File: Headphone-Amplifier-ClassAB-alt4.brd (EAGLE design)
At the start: 40.6 x 25.4 mm, 17 parts, among them T1 BC547, T2 BC557, T3 BC547

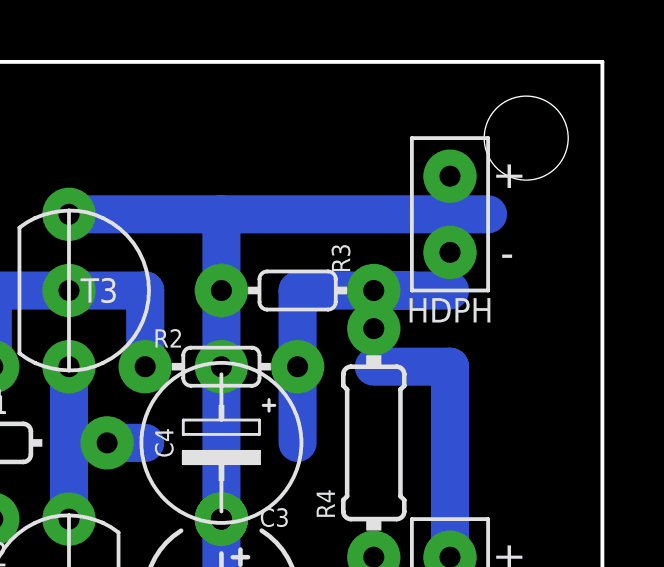
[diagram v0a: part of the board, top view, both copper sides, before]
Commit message: ...
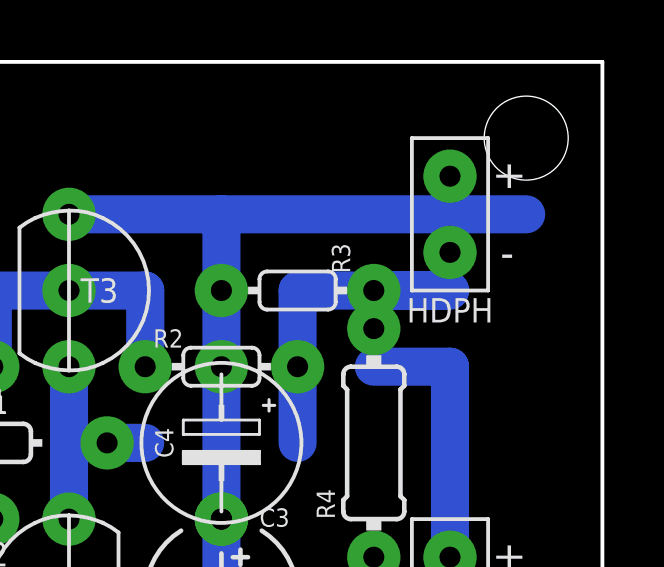
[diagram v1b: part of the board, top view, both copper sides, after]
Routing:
- net N$9: track 11.4 -> 12.7 mm
- net N$8: track 31.8 -> 33.0 mm
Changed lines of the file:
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@@
           <wire x1="30.48" y1="15.24" x2="30.48" y2="17.78" width="1.27" layer="16" />
           <wire x1="30.48" y1="17.78" x2="33.02" y2="17.78" width="1.27" layer="16" />
-          <wire x1="34.29" y1="17.78" x2="33.02" y2="17.78" width="1.27" layer="16" />
+          <wire x1="35.56" y1="17.78" x2="33.02" y2="17.78" width="1.27" layer="16" />
           <wire x1="33.02" y1="17.78" x2="35.56" y2="17.78" width="1.27" layer="16" />
           <wire x1="30.48" y1="15.24" x2="30.48" y2="12.7" width="1.27" layer="16" />
@@
           <wire x1="27.94" y1="20.32" x2="22.86" y2="20.32" width="1.27" layer="16" />
           <wire x1="27.94" y1="20.32" x2="35.56" y2="20.32" width="1.27" layer="16" />
-          <wire x1="35.56" y1="20.32" x2="36.83" y2="20.32" width="1.27" layer="16" />
+          <wire x1="35.56" y1="20.32" x2="38.1" y2="20.32" width="1.27" layer="16" />
         </signal>
         <signal name="V+">

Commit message: ...
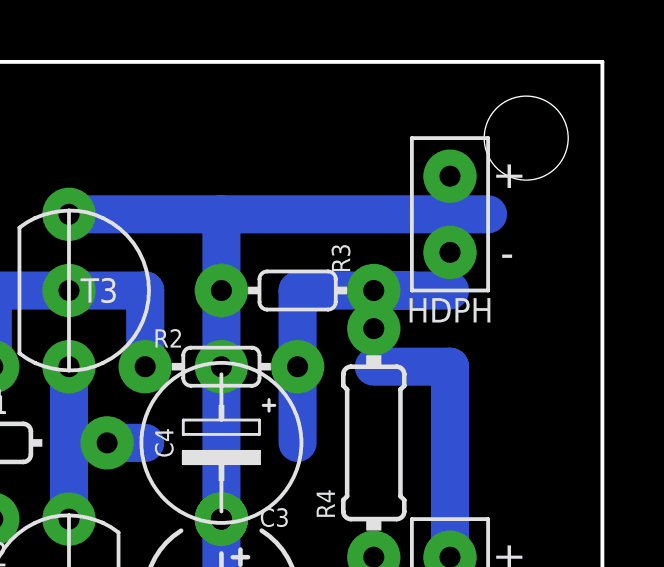
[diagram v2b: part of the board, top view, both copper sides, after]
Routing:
- net N$9: track 12.7 -> 11.4 mm
- net N$8: track 33.0 -> 31.8 mm
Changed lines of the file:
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@@
           <wire x1="30.48" y1="15.24" x2="30.48" y2="17.78" width="1.27" layer="16" />
           <wire x1="30.48" y1="17.78" x2="33.02" y2="17.78" width="1.27" layer="16" />
-          <wire x1="35.56" y1="17.78" x2="33.02" y2="17.78" width="1.27" layer="16" />
+          <wire x1="34.29" y1="17.78" x2="33.02" y2="17.78" width="1.27" layer="16" />
           <wire x1="33.02" y1="17.78" x2="35.56" y2="17.78" width="1.27" layer="16" />
           <wire x1="30.48" y1="15.24" x2="30.48" y2="12.7" width="1.27" layer="16" />
@@
           <wire x1="27.94" y1="20.32" x2="22.86" y2="20.32" width="1.27" layer="16" />
           <wire x1="27.94" y1="20.32" x2="35.56" y2="20.32" width="1.27" layer="16" />
-          <wire x1="35.56" y1="20.32" x2="38.1" y2="20.32" width="1.27" layer="16" />
+          <wire x1="35.56" y1="20.32" x2="36.83" y2="20.32" width="1.27" layer="16" />
         </signal>
         <signal name="V+">

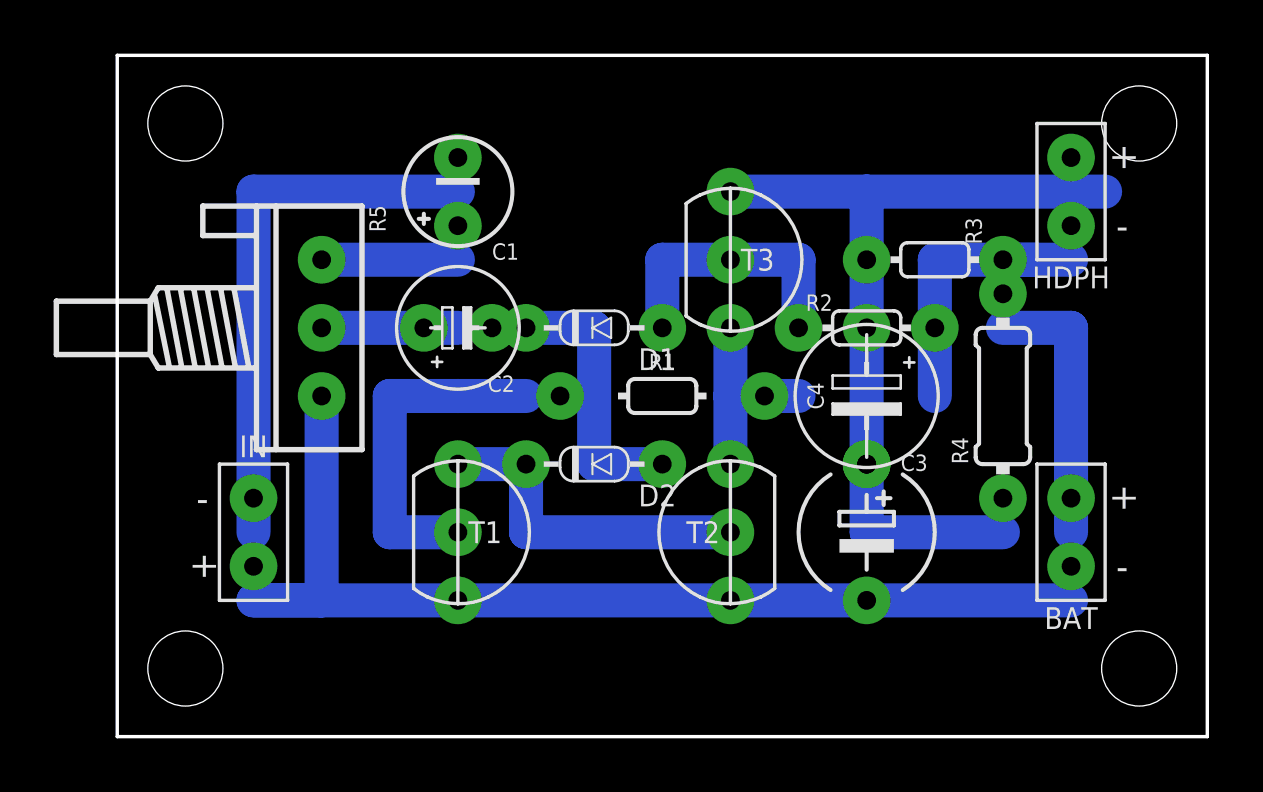
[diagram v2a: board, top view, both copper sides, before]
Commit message: ...
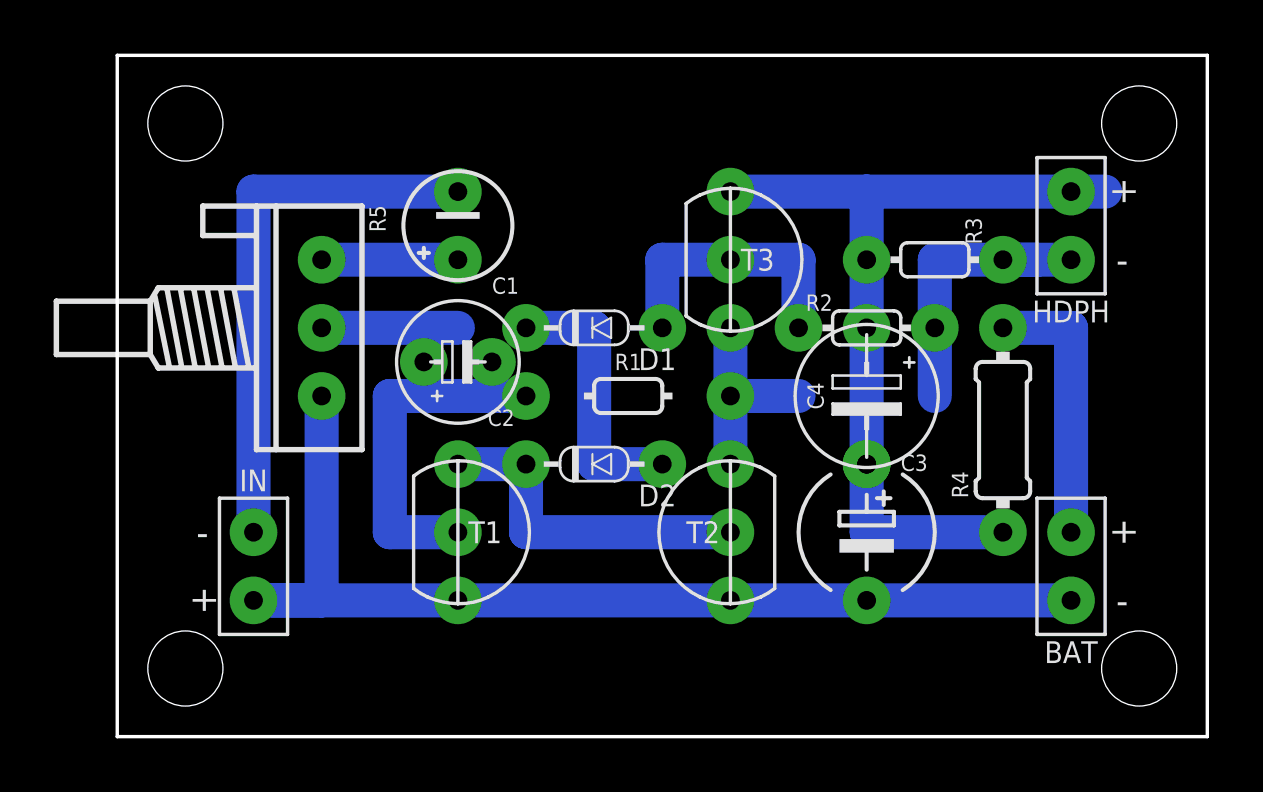
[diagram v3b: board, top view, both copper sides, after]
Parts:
- moved BAT 1.27 mm to (35.6, 6.35)
- moved IN 1.27 mm to (5.08, 6.35)
- moved C1 1.27 mm to (12.7, 19.1)
- moved C2 1.27 mm to (12.7, 14.0)
- moved HDPH 1.27 mm to (35.6, 19.1)
- moved R1 1.27 mm to (19.1, 12.7)
- moved R4 1.27 mm to (33.0, 11.4)
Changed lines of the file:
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@@
       <setting verticaltext="up" />
     </settings>
-    <grid distance="50" unitdist="mil" unit="mil" style="dots" multiple="2" display="yes" altdistance="25" altunitdist="mil" altunit="mil" />
+    <grid distance="0.05" unitdist="inch" unit="inch" style="dots" multiple="2" display="yes" altdistance="0.005" altunitdist="inch" altunit="inch" />
     <layers>
       <layer number="1" name="Top" color="4" fill="1" visible="yes" active="yes" />
-      <layer number="2" name="Route2" color="1" fill="3" visible="no" active="no" />
-      <layer number="3" name="Route3" color="4" fill="3" visible="no" active="no" />
-      <layer number="4" name="Route4" color="1" fill="4" visible="no" active="no" />
-      <layer number="5" name="Route5" color="4" fill="4" visible="no" active="no" />
-      <layer number="6" name="Route6" color="1" fill="8" visible="no" active="no" />
-      <layer number="7" name="Route7" color="4" fill="8" visible="no" active="no" />
-      <layer number="8" name="Route8" color="1" fill="2" visible="no" active="no" />
-      <layer number="9" name="Route9" color="4" fill="2" visible="no" active="no" />
-      <layer number="10" name="Route10" color="1" fill="7" visible="no" active="no" />
-      <layer number="11" name="Route11" color="4" fill="7" visible="no" active="no" />
-      <layer number="12" name="Route12" color="1" fill="5" visible="no" active="no" />
-      <layer number="13" name="Route13" color="4" fill="5" visible="no" active="no" />
-      <layer number="14" name="Route14" color="1" fill="6" visible="no" active="no" />
-      <layer number="15" name="Route15" color="4" fill="6" visible="no" active="no" />
       <layer number="16" name="Bottom" color="1" fill="1" visible="yes" active="yes" />
       <layer number="17" name="Pads" color="2" fill="1" visible="yes" active="yes" />
       <layer number="18" name="Vias" color="2" fill="1" visible="yes" active="yes" />
       <layer number="19" name="Unrouted" color="6" fill="1" visible="yes" active="yes" />
-      <layer number="20" name="Dimension" color="15" fill="1" visible="yes" active="yes" />
-      <layer number="21" name="tPlace" color="7" fill="1" visible="yes" active="yes" />
-      <layer number="22" name="bPlace" color="7" fill="1" visible="yes" active="yes" />
+      <layer number="20" name="Dimension" color="24" fill="1" visible="yes" active="yes" />
+      <layer number="21" name="tPlace" color="16" fill="1" visible="yes" active="yes" />
+      <layer number="22" name="bPlace" color="14" fill="1" visible="yes" active="yes" />
       <layer number="23" name="tOrigins" color="15" fill="1" visible="yes" active="yes" />
       <layer number="24" name="bOrigins" color="15" fill="1" visible="yes" active="yes" />
@@
       <layer number="37" name="tTest" color="7" fill="1" visible="no" active="yes" />
       <layer number="38" name="bTest" color="7" fill="1" visible="no" active="yes" />
-      <layer number="39" name="tKeepout" color="4" fill="11" visible="yes" active="yes" />
-      <layer number="40" name="bKeepout" color="1" fill="11" visible="yes" active="yes" />
-      <layer number="41" name="tRestrict" color="4" fill="10" visible="yes" active="yes" />
-      <layer number="42" name="bRestrict" color="1" fill="10" visible="yes" active="yes" />
-      <layer number="43" name="vRestrict" color="2" fill="10" visible="yes" active="yes" />
+      <layer number="39" name="tKeepout" color="4" fill="11" visible="no" active="yes" />
+      <layer number="40" name="bKeepout" color="1" fill="11" visible="no" active="yes" />
+      <layer number="41" name="tRestrict" color="4" fill="10" visible="no" active="yes" />
+      <layer number="42" name="bRestrict" color="1" fill="10" visible="no" active="yes" />
+      <layer number="43" name="vRestrict" color="2" fill="10" visible="no" active="yes" />
       <layer number="44" name="Drills" color="7" fill="1" visible="no" active="yes" />
       <layer number="45" name="Holes" color="7" fill="1" visible="yes" active="yes" />
       <layer number="46" name="Milling" color="3" fill="1" visible="no" active="yes" />
       <layer number="47" name="Measures" color="7" fill="1" visible="no" active="yes" />
-      <layer number="48" name="Document" color="7" fill="1" visible="yes" active="yes" />
-      <layer number="49" name="Reference" color="7" fill="1" visible="yes" active="yes" />
-      <layer number="51" name="tDocu" color="7" fill="1" visible="yes" active="yes" />
-      <layer number="52" name="bDocu" color="7" fill="1" visible="yes" active="yes" />
-      <layer number="90" name="Modules" color="5" fill="1" visible="no" active="no" />
+      <layer number="48" name="Document" color="7" fill="1" visible="no" active="yes" />
+      <layer number="49" name="Reference" color="7" fill="1" visible="no" active="yes" />
+      <layer number="51" name="tDocu" color="6" fill="1" visible="yes" active="yes" />
+      <layer number="52" name="bDocu" color="7" fill="1" visible="no" active="yes" />
       <layer number="91" name="Nets" color="2" fill="1" visible="no" active="no" />
       <layer number="92" name="Busses" color="1" fill="1" visible="no" active="no" />
@@
       <layer number="95" name="Names" color="7" fill="1" visible="no" active="no" />
       <layer number="96" name="Values" color="7" fill="1" visible="no" active="no" />
+      <layer number="2" name="Route2" color="1" fill="3" visible="no" active="no" />
+      <layer number="3" name="Route3" color="4" fill="3" visible="no" active="no" />
+      <layer number="4" name="Route4" color="1" fill="4" visible="no" active="no" />
+      <layer number="5" name="Route5" color="4" fill="4" visible="no" active="no" />
+      <layer number="6" name="Route6" color="1" fill="8" visible="no" active="no" />
+      <layer number="7" name="Route7" color="4" fill="8" visible="no" active="no" />
+      <layer number="8" name="Route8" color="1" fill="2" visible="no" active="no" />
+      <layer number="9" name="Route9" color="4" fill="2" visible="no" active="no" />
+      <layer number="10" name="Route10" color="1" fill="7" visible="no" active="no" />
+      <layer number="11" name="Route11" color="4" fill="7" visible="no" active="no" />
+      <layer number="12" name="Route12" color="1" fill="5" visible="no" active="no" />
+      <layer number="13" name="Route13" color="4" fill="5" visible="no" active="no" />
+      <layer number="14" name="Route14" color="1" fill="6" visible="no" active="no" />
+      <layer number="15" name="Route15" color="4" fill="6" visible="no" active="no" />
+      <layer number="90" name="Modules" color="5" fill="1" visible="no" active="no" />
       <layer number="97" name="Info" color="7" fill="1" visible="no" active="no" />
       <layer number="98" name="Guide" color="6" fill="1" visible="no" active="no" />
       <layer number="99" name="SpiceOrder" color="7" fill="1" visible="no" active="no" />
-      <layer number="250" name="trash" color="7" fill="1" visible="yes" active="yes" />
+      <layer number="250" name="trash" color="7" fill="1" visible="no" active="no" />
     </layers>
     <board>
@@
       </autorouter>
       <elements>
-        <element name="BAT" library="pad" package="SPAD+-" value="SPAD+-+-" x="35.56" y="7.62" />
-        <element name="C1" library="c" package="E2.5-4/V" value="4.7uF" x="12.7" y="20.32" rot="R180" />
-        <element name="C2" library="c" package="E2,5-4" value="4.7uF" x="12.7" y="15.24" rot="R180" />
+        <element name="BAT" library="pad" package="SPAD+-" value="SPAD+-+-" x="35.56" y="6.35" />
+        <element name="C1" library="c" package="E2.5-4/V" value="4.7uF" x="12.7" y="19.05" rot="R180" />
+        <element name="C2" library="c" package="E2,5-4" value="4.7uF" x="12.7" y="13.97" rot="R180" />
         <element name="C3" library="c" package="E5-5/V" value="100-1000uF" x="27.94" y="7.62" />
         <element name="C4" library="c" package="E5-4" value="220uF" x="27.94" y="12.7" rot="R270" />
         <element name="D1" library="d" package="DO34-5" value="1N4148" x="17.78" y="15.24" />
         <element name="D2" library="d" package="DO34-5" value="1N4148" x="17.78" y="10.16" />
-        <element name="HDPH" library="pad" package="SPAD+-" value="SPAD+-+-" x="35.56" y="20.32" />
-        <element name="IN" library="pad" package="SPAD+-" value="SPAD+-+-" x="5.08" y="7.62" rot="R180" />
-        <element name="R1" library="r" package="0202/7" value="100k" x="20.32" y="12.7" />
+        <element name="HDPH" library="pad" package="SPAD+-" value="SPAD+-+-" x="35.56" y="19.05" />
+        <element name="IN" library="pad" package="SPAD+-" value="SPAD+-+-" x="5.08" y="6.35" rot="R180" />
+        <element name="R1" library="r" package="0202/7" value="100k" x="19.05" y="12.7" />
         <element name="R2" library="r" package="0202/5" value="330" x="27.94" y="15.24" />
         <element name="R3" library="r" package="0202/5-V" value="100" x="30.48" y="17.78" rot="R270" />
-        <element name="R4" library="r" package="0204/7" value="22" x="33.02" y="12.7" rot="R90" />
+        <element name="R4" library="r" package="0204/7" value="22" x="33.02" y="11.43" rot="R90" />
         <element name="R5" library="r" package="POT" value="100k" x="7.62" y="15.24" rot="R270" />
         <element name="T1" library="t" package="TO92-CBE" value="BC547" x="12.7" y="7.62" />
